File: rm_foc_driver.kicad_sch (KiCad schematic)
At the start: 66 parts, among them J1 TMC4671, J2 Conn_01x02, J3 Conn_01x03, J4 Conn_01x03, Q1 CSD18540Q5B, Q2 CSD18540Q5B, Q3 CSD18540Q5B, Q4 CSD18540Q5B, Q5 CSD18540Q5B, Q6 CSD18540Q5B, U1 TPS54540, U10 74HC244, U2 SY8303, U3 IR2104, U4 IR2104, U5 IR2104, U6 LM236, U7 LM236, U8 INA199, U9 INA199

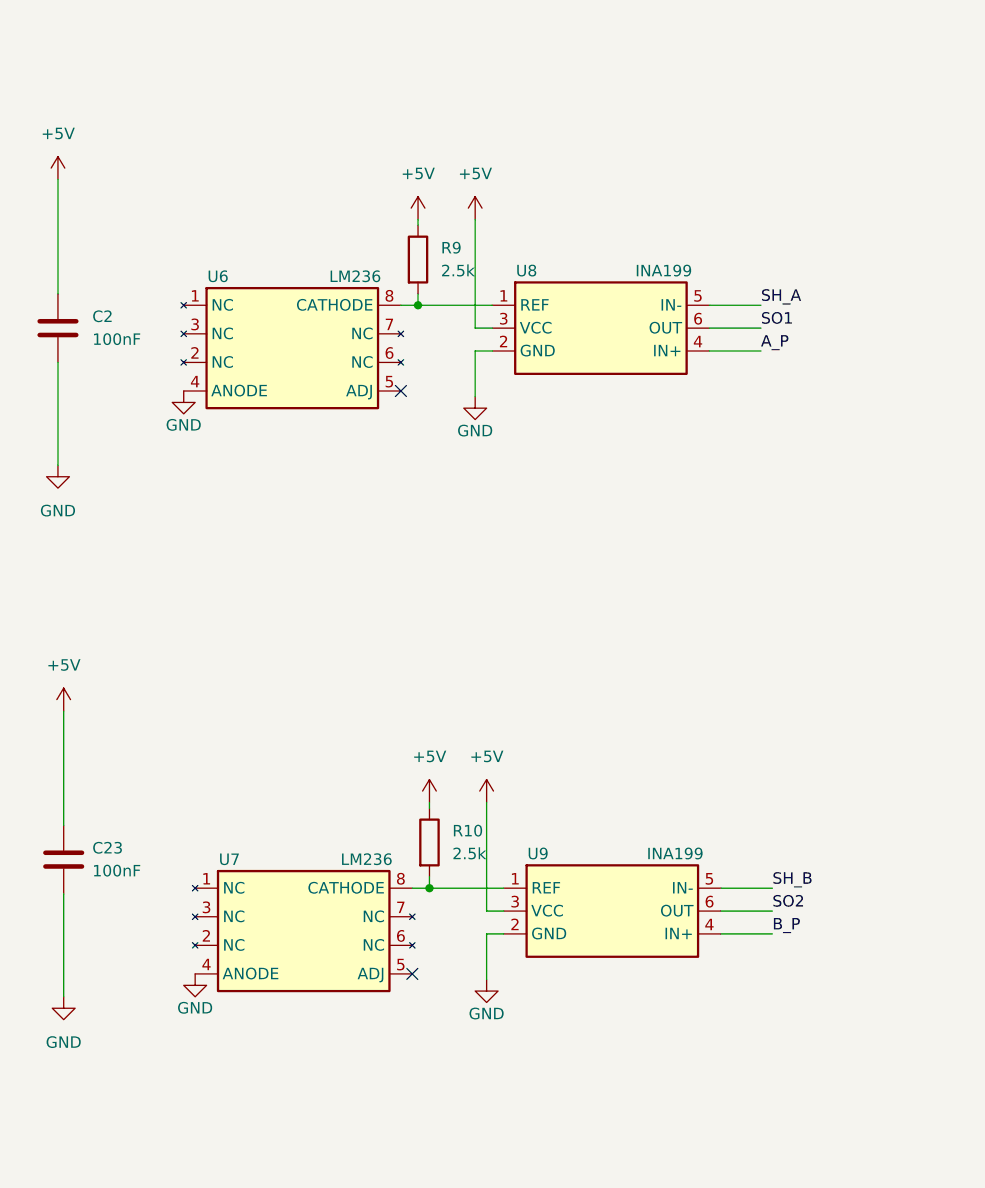
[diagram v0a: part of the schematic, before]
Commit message: 20230111 AD8418
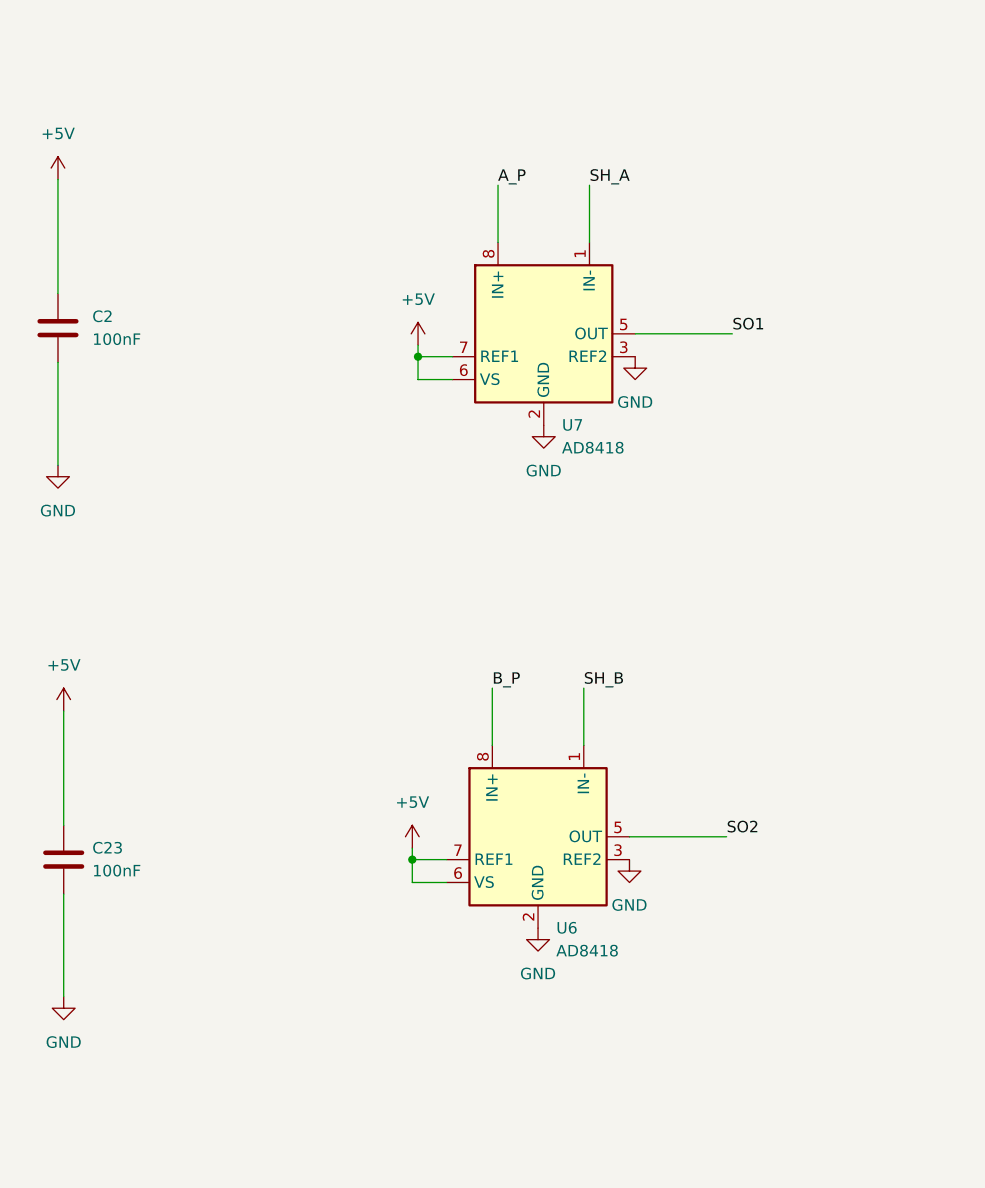
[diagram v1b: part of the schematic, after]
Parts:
- removed R10, R9: 2.5k, Resistor_SMD:R_0603_1608Metric, symbol Device:R
- removed U6, U7: LM236, Package_SO:PowerIntegrations_SO-8, symbol My_lib:LM236
- removed U8, U9: INA199, Package_TO_SOT_SMD:SOT-363_SC-70-6_Handsoldering, symbol My_lib:INA199
- added U6, U7: AD8418, Package_SO:SOP-8_3.9x4.9mm_P1.27mm, symbol Amplifier_Current:AD8418
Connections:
- net +5V: now also U6.6 (VS), U6.7 (REF1), U7.6 (VS), U7.7 (REF1)
- net A_P: now also U7.8 (IN+)
- net B_P: now also U6.8 (IN+)
- net GND: now also U6.2 (GND), U6.3 (REF2), U7.2 (GND), U7.3 (REF2)
- net SH_A: now also U7.1 (IN-)
- net SH_B: now also U6.1 (IN-)
- net SO1: now also U7.5 (OUT)
- net SO2: now also U6.5 (OUT)
- no-connect marks 14 -> 12
